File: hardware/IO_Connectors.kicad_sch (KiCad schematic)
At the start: 20 parts, among them J3 USB_B_Micro

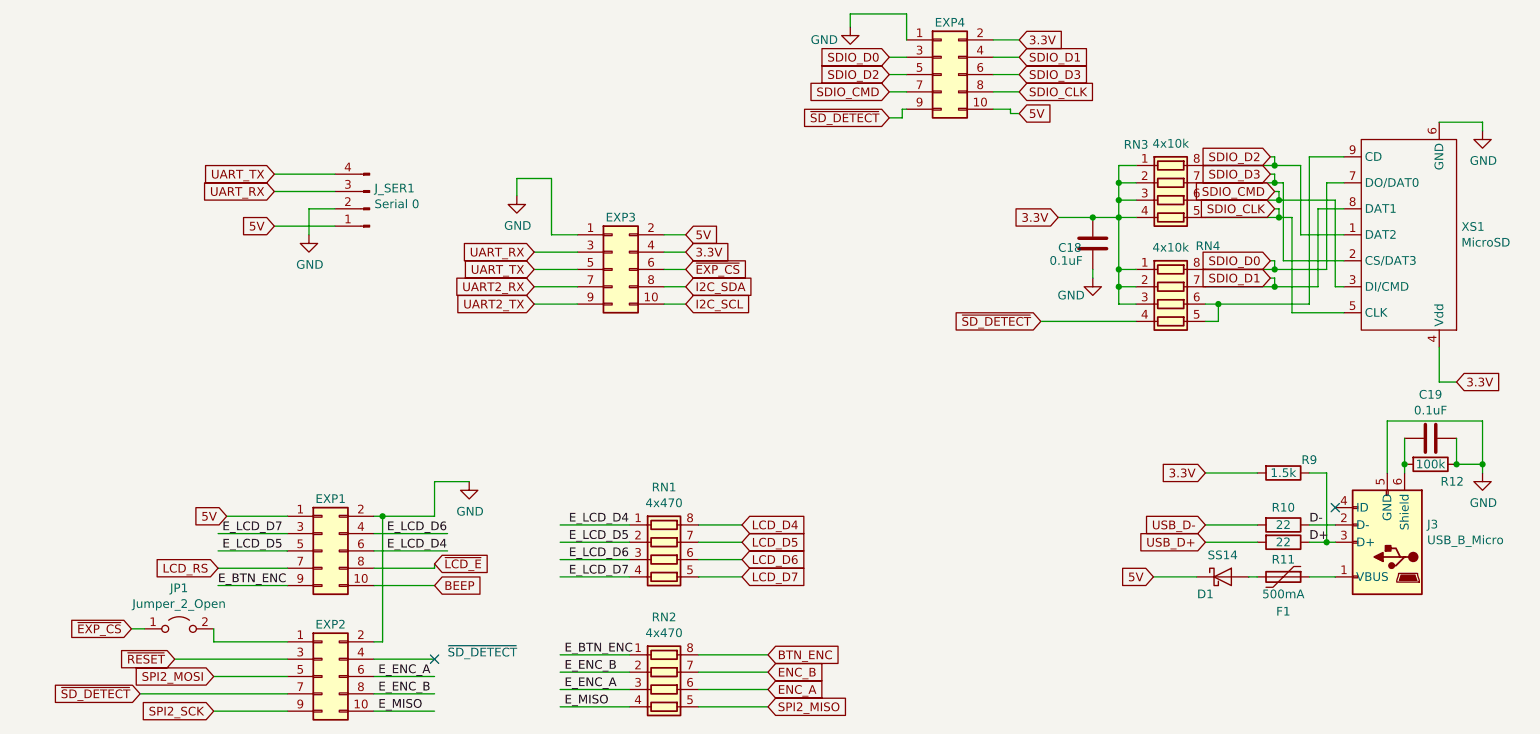
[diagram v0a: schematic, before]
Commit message: Update PrntrBoard fabrication files.
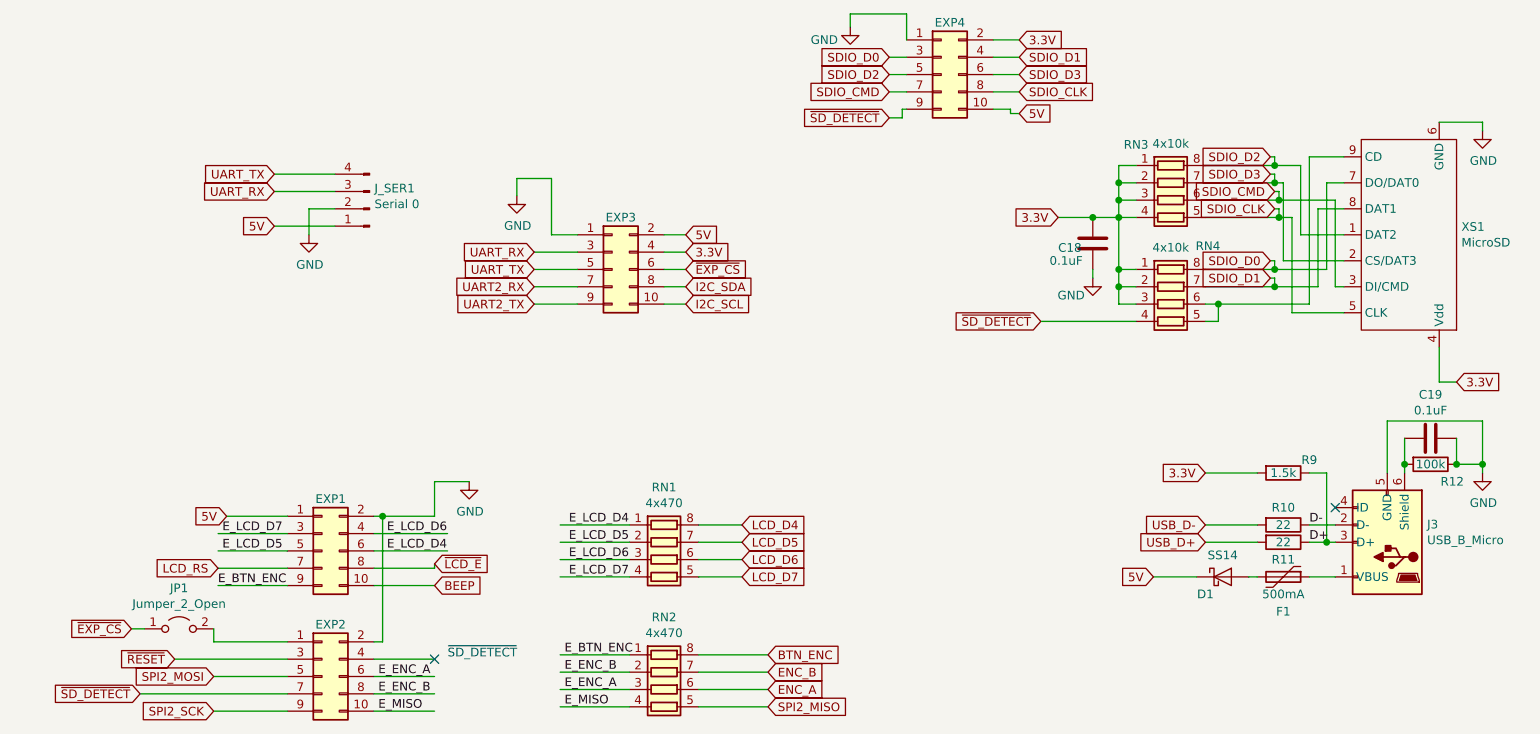
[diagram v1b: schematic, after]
